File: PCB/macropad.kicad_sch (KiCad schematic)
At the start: 11 parts, among them SW1 SW_Push, SW2 SW_Push, SW3 SW_Push, SW4 SW_Push, SW5 SW_Push, SW6 SW_Push, SW7 SW_Push, SW8 SW_Push, SW9 SW_Push, U1 XIAO-RP2040-DIP

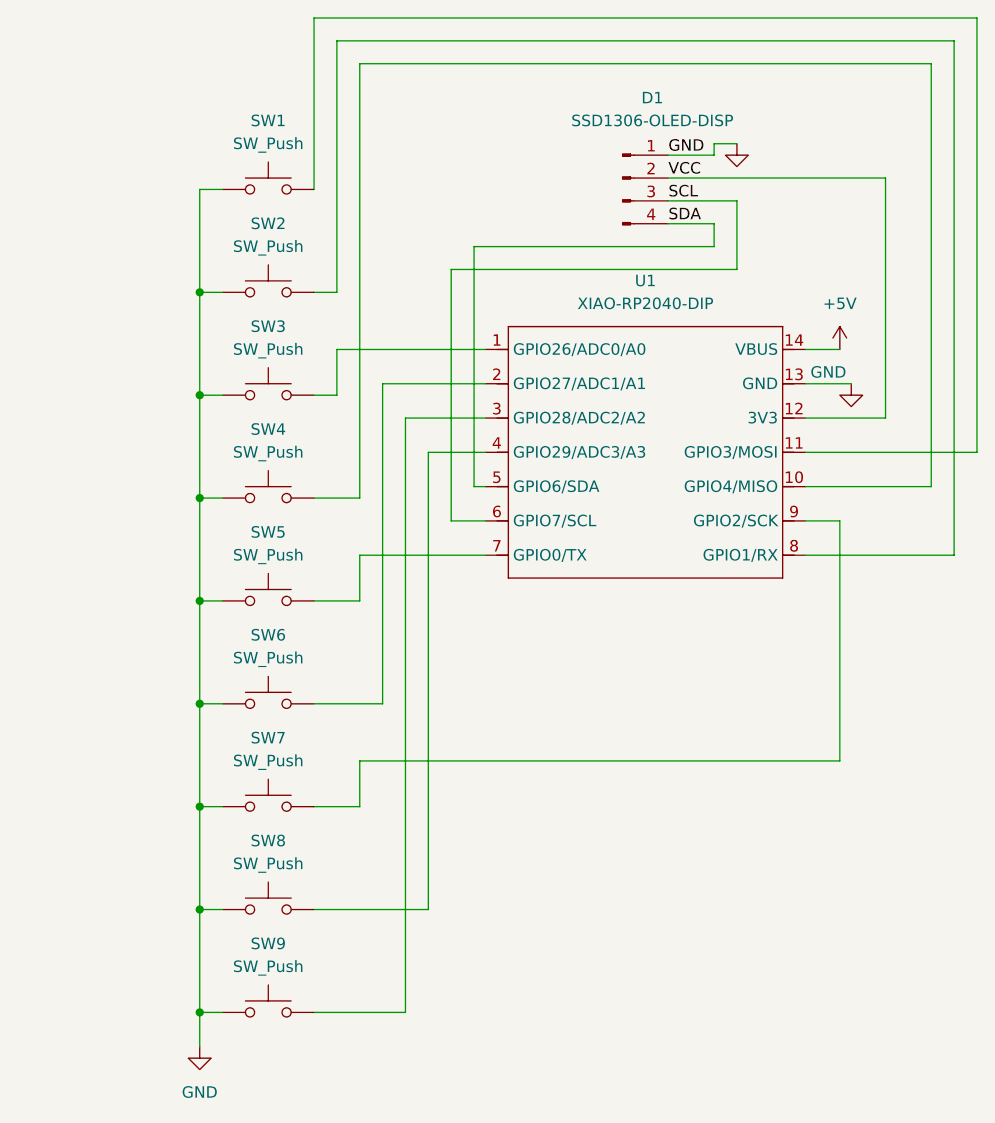
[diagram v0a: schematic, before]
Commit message: PCB v.2
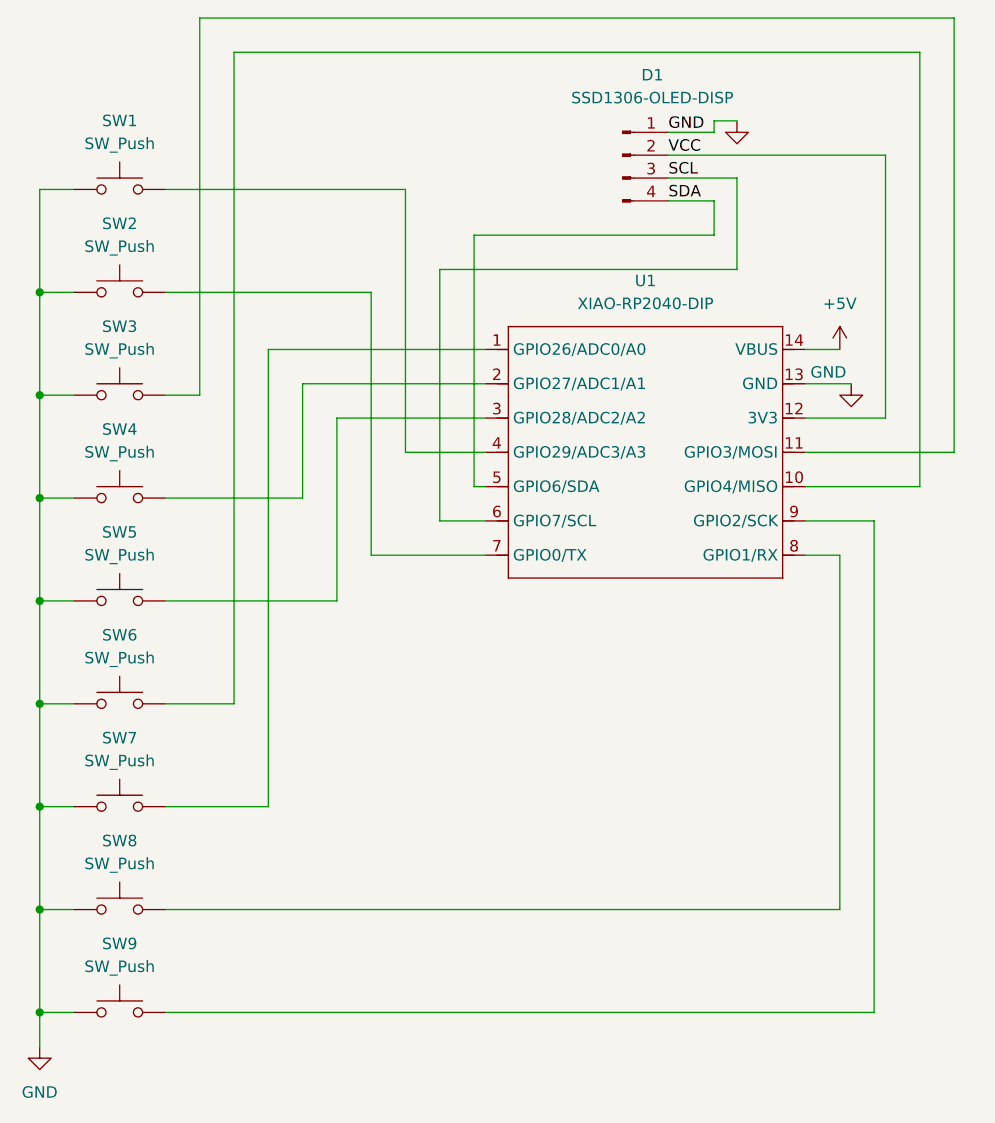
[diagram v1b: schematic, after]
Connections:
- net at SW3.2: now also U1.11 (GPIO3/MOSI); no longer U1.1 (GPIO26/ADC0/A0)
- net at SW7.2: now also U1.1 (GPIO26/ADC0/A0); no longer U1.9 (GPIO2/SCK)
- net at SW5.2: now also U1.3 (GPIO28/ADC2/A2); no longer U1.7 (GPIO0/TX)
- net at SW6.2: now also U1.10 (GPIO4/MISO); no longer U1.2 (GPIO27/ADC1/A1)
- net at SW2.2: now also U1.7 (GPIO0/TX); no longer U1.8 (GPIO1/RX)
- net at SW8.2: now also U1.8 (GPIO1/RX); no longer U1.4 (GPIO29/ADC3/A3)
- net at SW1.2: now also U1.4 (GPIO29/ADC3/A3); no longer U1.11 (GPIO3/MOSI)
- net at SW4.2: now also U1.2 (GPIO27/ADC1/A1); no longer U1.10 (GPIO4/MISO)
- net at SW9.2: now also U1.9 (GPIO2/SCK); no longer U1.3 (GPIO28/ADC2/A2)
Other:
- moved on the sheet: D1, SW1, SW2, SW3, SW4, SW5, SW6, SW7, SW8, SW9
